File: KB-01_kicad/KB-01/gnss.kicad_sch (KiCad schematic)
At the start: 9 parts, among them U3 TESEO-LIV3F, U7 TLV70033_SOT353, U8 MAX2659ELT+T

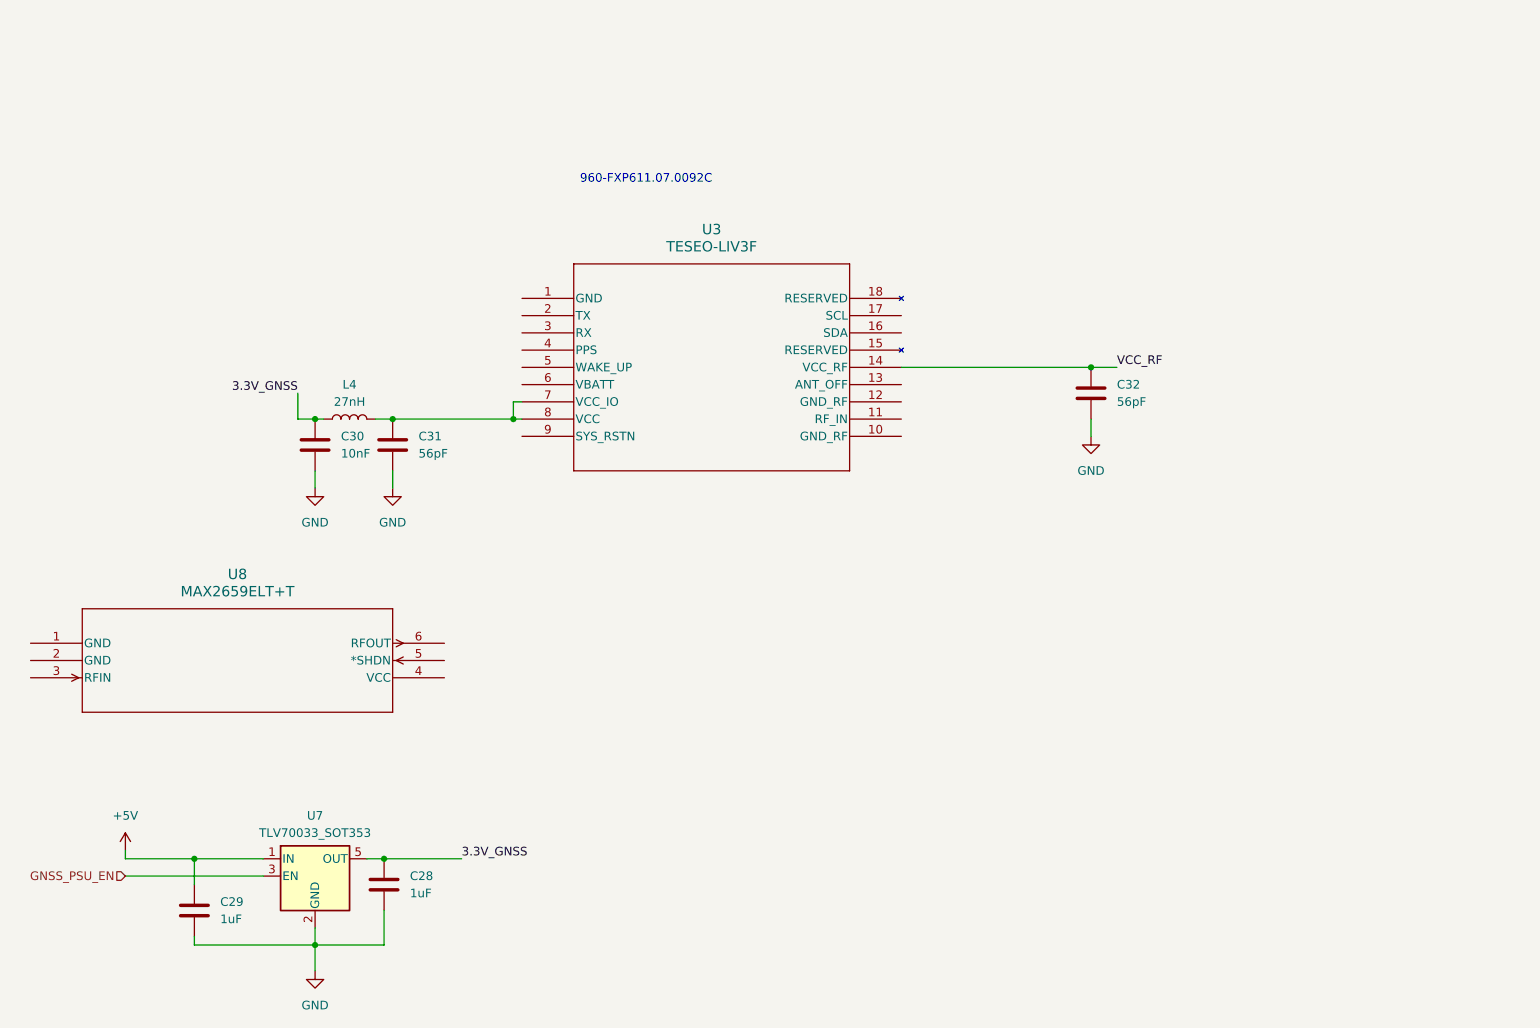
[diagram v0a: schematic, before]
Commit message: hi
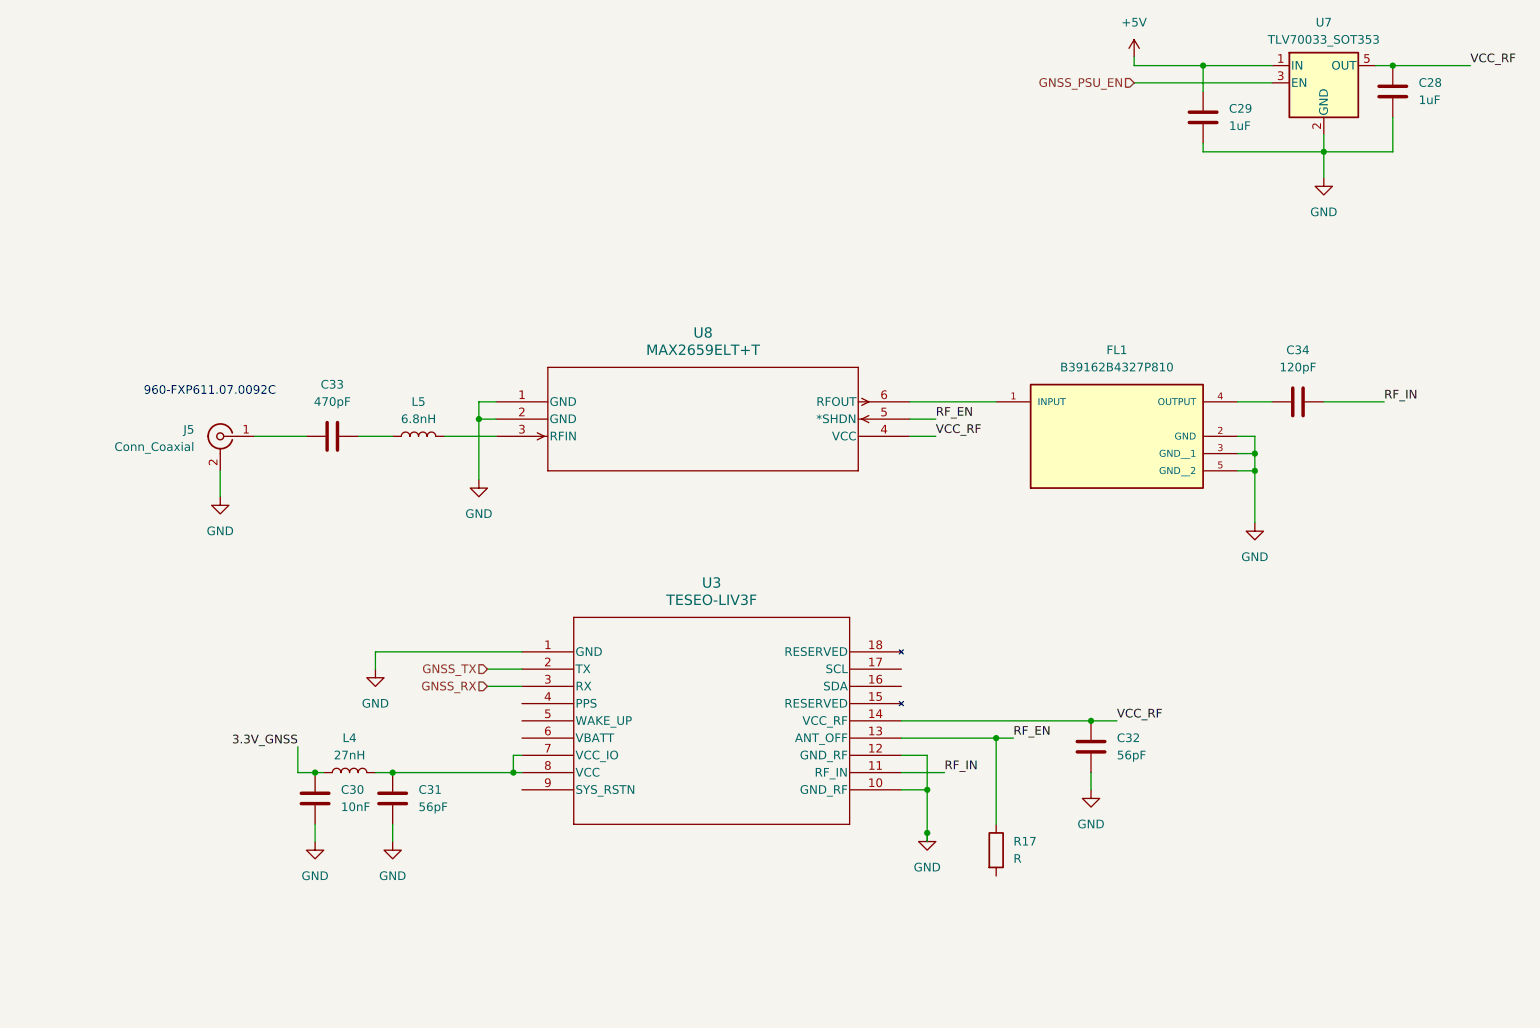
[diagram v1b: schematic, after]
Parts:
- added C33: 470pF, Capacitor_SMD:C_0402_1005Metric_Pad0.74x0.62mm_HandSolder, symbol Device:C
- added C34: 120pF, Capacitor_SMD:C_0402_1005Metric_Pad0.74x0.62mm_HandSolder, symbol Device:C
- added FL1: B39162B4327P810, B39162B4327P810:FIL_B39162B4327P810, symbol B39162B4327P810:B39162B4327P810
- added J5: Conn_Coaxial, Connector_Coaxial:U.FL_Hirose_U.FL-R-SMT-1_Vertical, symbol Connector:Conn_Coaxial
- added L5: 6.8nH, Inductor_SMD:L_0402_1005Metric_Pad0.77x0.64mm_HandSolder, symbol Device:L
- added R17: R, Resistor_SMD:R_0402_1005Metric_Pad0.72x0.64mm_HandSolder, symbol Device:R
- U8: footprint 21-0147-L611+2_MXM -> footprints:21-0147-L611&plus_2_MXM
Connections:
- net 3.3V_GNSS: no longer C28.1, U7.5 (OUT)
- net GND: now also U3.1 (GND), U3.10 (GND_RF), U3.12 (GND_RF), U8.1 (GND), U8.2 (GND), FL1.2 (GND), FL1.3 (GND__1), FL1.5 (GND__2), J5.2 (Ext)
- net VCC_RF: now also C28.1, U7.5 (OUT), U8.4 (VCC)
- net RF_IN: now reaches U3.11 (RF_IN)
- net RF_IN: now also C34.2
- net RF_EN: now reaches U3.13 (ANT_OFF)
- net RF_EN: now also U8.5 (*SHDN), R17.1
- net GNSS_TX: now reaches U3.2 (TX)
- net GNSS_RX: now reaches U3.3 (RX)
- net at U8.3 (RFIN): now also L5.2
- net at U8.6 (RFOUT): now also FL1.1 (INPUT)
- new net: C33.1, J5.1 (In)
- new net: C33.2, L5.1
- new net: C34.1, FL1.4 (OUTPUT)
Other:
- moved on the sheet: C28, C29, C30, C31, C32, L4, U3, U7, U8
